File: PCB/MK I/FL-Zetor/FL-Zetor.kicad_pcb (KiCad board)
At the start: 2 copper layers, 120 x 65 mm, 24 parts, among them J1 Conn_01x02_Pin, J2 Conn_01x06_Pin, J3 Conn_01x06_Pin, J4 Conn_01x06_Pin, J5 Conn_01x06_Pin, SW1 SL19, U1 TSOP382xx, U2 LM1086

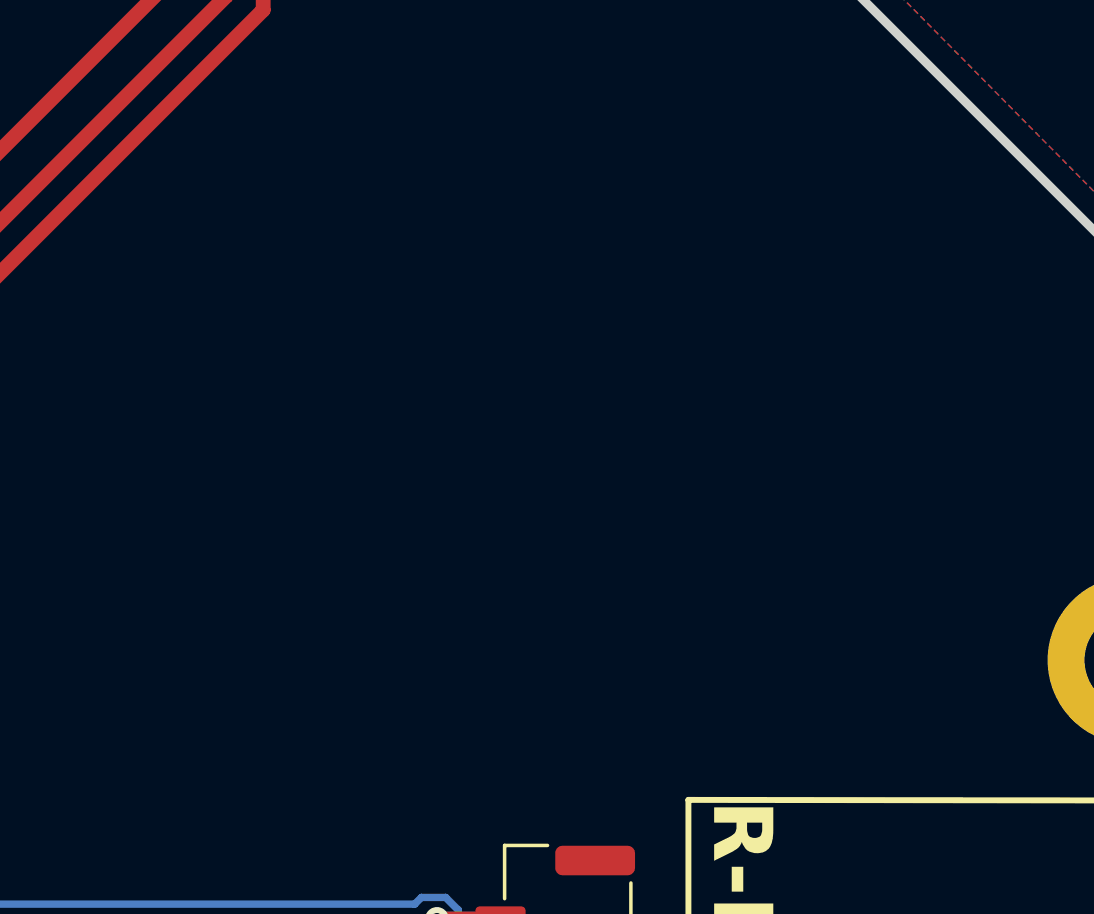
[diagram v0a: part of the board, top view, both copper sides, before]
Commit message: some shit
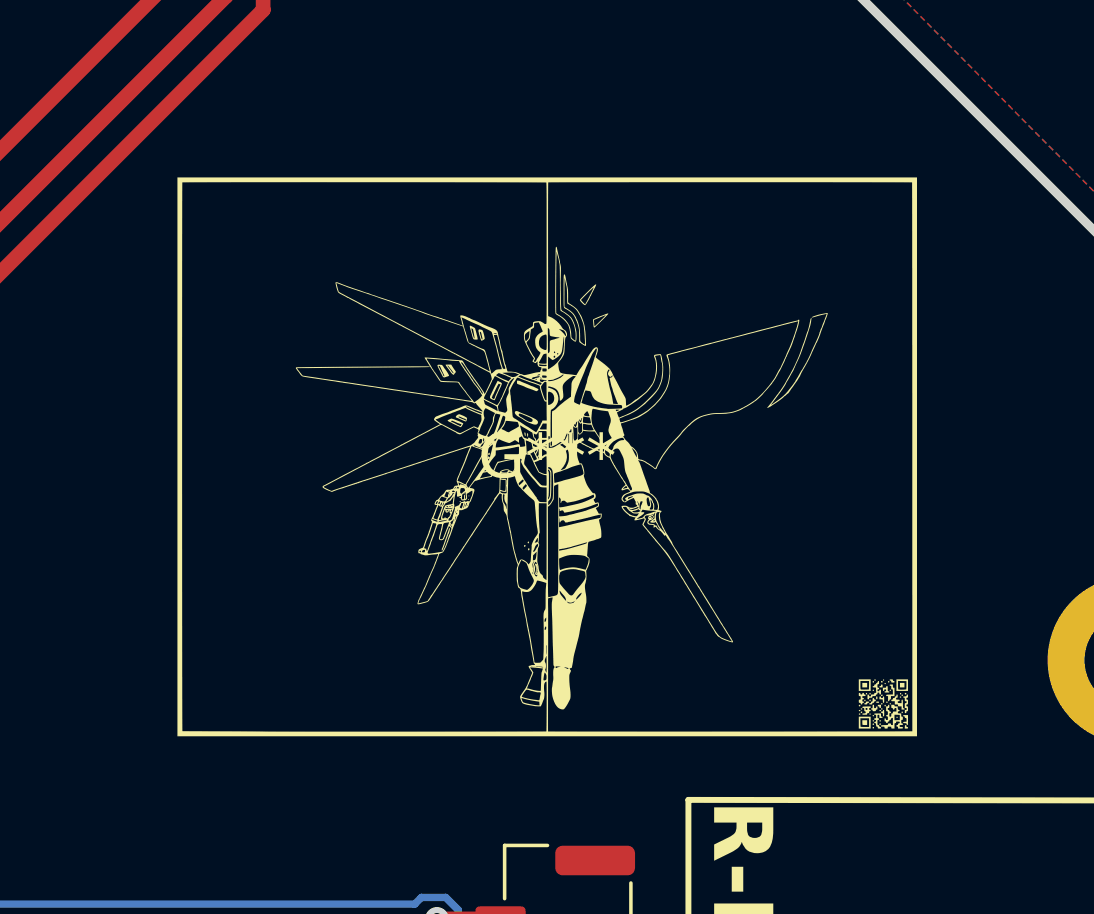
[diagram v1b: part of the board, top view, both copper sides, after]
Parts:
- added G***: LOGO, LOGO, F.Cu at (184.6, 93.9)
